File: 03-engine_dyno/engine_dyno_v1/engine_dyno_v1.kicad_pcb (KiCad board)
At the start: 4 copper layers, 92 parts, among them J1 Screw_Terminal_01x02, J2 Screw_Terminal_01x02, J3 Screw_Terminal_01x02, J4 Screw_Terminal_01x05, J5 Screw_Terminal_01x03, J6 Screw_Terminal_01x05, J7 Screw_Terminal_01x03, P1 J1B1211CCD, Q1 PMOS, U1 LMR51430XDDCR, U10 INA827AIDGKR, U11 74LVC1G17, U12 AD630ARZ, U13 ADS1120IPWR, U14 OPA192IDBVR, U15 OPA192IDBVR, U16 74LVC1G17, U2 TVS1800DRV, U3 TPS2115APWR, U4 TPS60403DBVRG4, U5 AD5689RBRUZ, U6 Teensy4.1, U7 INA827AIDGKR, U8 AD630ARZ, U9 ADS1120IPWR

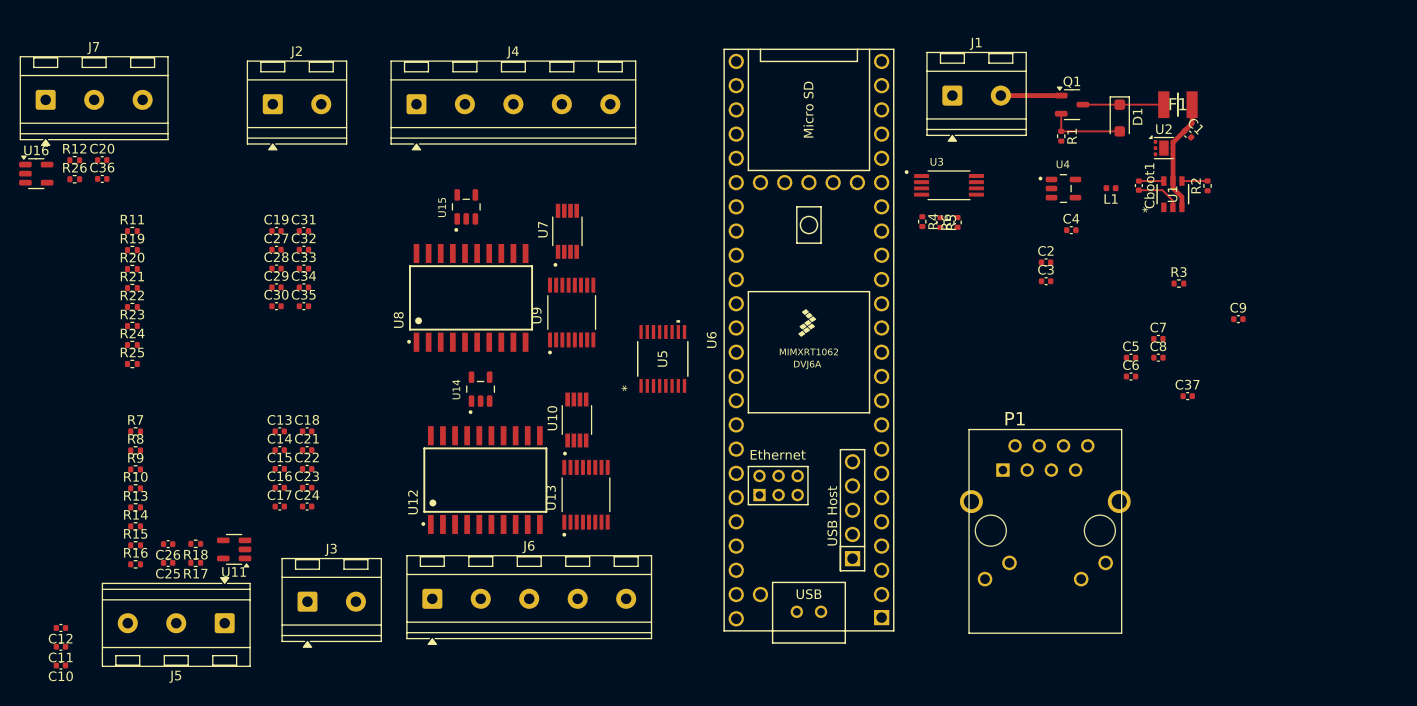
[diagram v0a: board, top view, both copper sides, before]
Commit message: some more changes
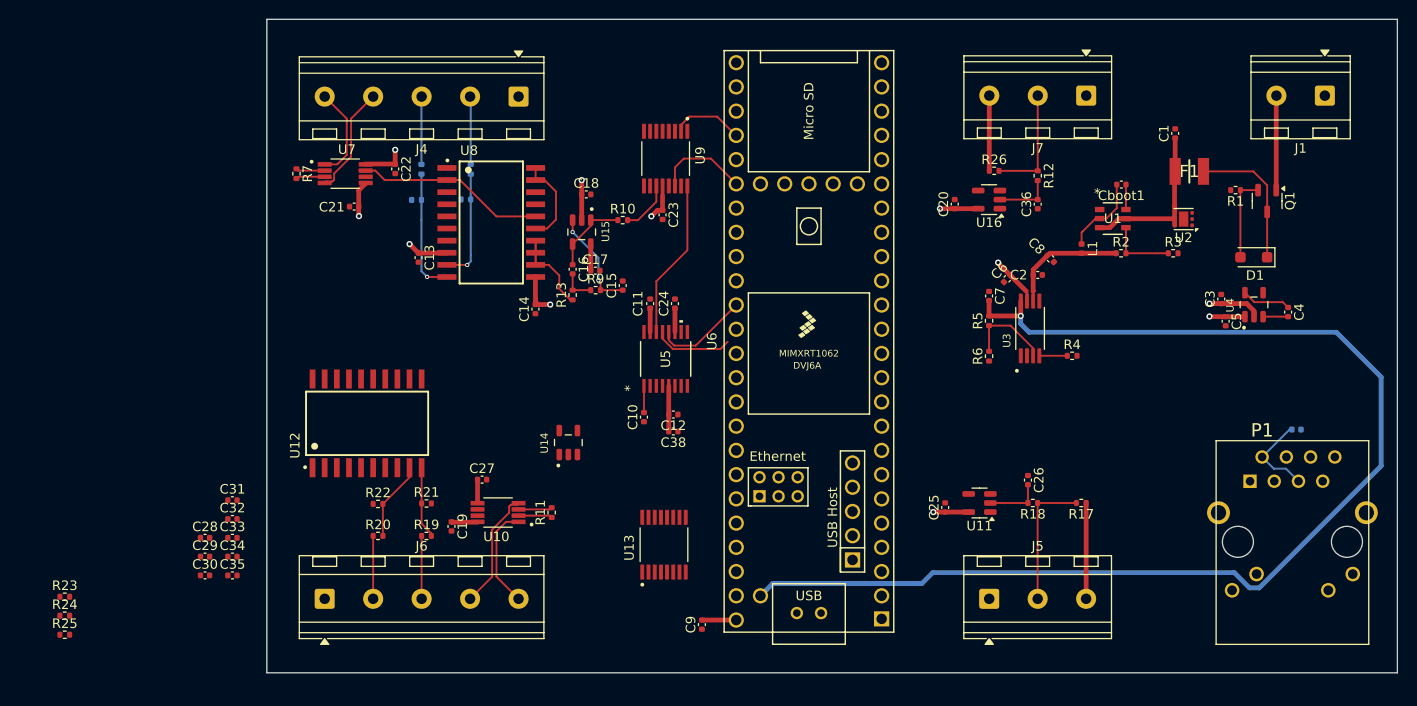
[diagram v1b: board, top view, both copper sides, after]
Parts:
- removed J2, J3: Screw_Terminal_01x02, TerminalBlock_RND:TerminalBlock_RND_205-00232_1x02_P5.08mm_Horizontal
- added C38: 10u, Capacitor_SMD:C_0402_1005Metric, F.Cu at (137.0, 99.0)
- C37, R14, R15, R16, R8: moved to B.Cu
- R11: value 100 -> 390
- R7: value 390 -> 1.5k
- moved J7 109.1 mm to (180.3, 63.8), turned to 180 degrees
- moved R12 101.0 mm to (175.2, 72.2), turned to -90 degrees
- moved U16 99.9 mm to (170.1, 74.7), turned to 180 degrees
- moved C36 98.1 mm to (175.2, 75.2), turned to 90 degrees
- moved R26 96.4 mm to (170.6, 71.7)
- moved R17 93.0 mm to (179.8, 106.5)
- moved C26 90.4 mm to (174.2, 104.1), turned to -90 degrees
- moved C20 89.5 mm to (166.5, 75.2), turned to 90 degrees
- moved R18 87.8 mm to (174.7, 106.5)
- moved C25 81.7 mm to (165.5, 107.0), turned to 90 degrees
- moved J5 80.2 mm to (170.1, 116.5), turned to 0 degrees
- moved U11 78.3 mm to (169.1, 106.5)
- moved C11 71.5 mm to (134.6, 85.6), turned to -90 degrees
- moved C12 68.0 mm to (137.0, 97.2)
- moved C10 66.4 mm to (133.9, 97.5), turned to 90 degrees
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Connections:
- U12 pad 15: /TMNR-5KM/AD630_OUT -> Net-(U12-CH_A-)
- U6 pad 11: unconnected-(U6-9_OUT1C-Pad11) -> /MCU/A16
- U6 pad 12: /MCU/CS_1 -> unconnected-(U6-10_CS_MQSR-Pad12)
- U6 pad 29: /MCU/CS_3 -> unconnected-(U6-37_CS-Pad29)
- U6 pad 31: /MCU/A15 -> unconnected-(U6-39_MISO1_OUT1A-Pad31)
- U6 pad 32: /MCU/A16 -> unconnected-(U6-40_A16-Pad32)
- U6 pad 37: unconnected-(U6-15_A1_RX3_SPDIF_IN-Pad37) -> /MCU/CS_1
- U6 pad 38: /Hall1/HALL -> unconnected-(U6-16_A2_RX4_SCL1-Pad38)
- U6 pad 39: /Hall2/HALL -> unconnected-(U6-17_A3_TX4_SDA1-Pad39)
- U6 pad 4: unconnected-(U6-2_OUT2-Pad4) -> /Hall1/HALL
- U6 pad 44: unconnected-(U6-22_A8_CTX1-Pad44) -> /MCU/A15
- U6 pad 45: unconnected-(U6-23_A9_CRX1_MCLK1-Pad45) -> /MCU/CS_3
- U6 pad 5: unconnected-(U6-3_LRCLK2-Pad5) -> /Hall2/HALL
- U8 pad 15: /Model1605/AD630_OUT -> Net-(U8-CH_A-)
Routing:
- net /MCU/+5V_USB: track 0.00 -> 128.7 mm, vias 0 -> 1
- net +5V: track 0.00 -> 56.1 mm, vias 0 -> 5
- net Net-(U7-VOUT): track 0.00 -> 20.5 mm
- net -5V: track 0.00 -> 18.4 mm, vias 0 -> 4
- net /MCU/MOSI: track 0.00 -> 16.7 mm
- net /Hall2/SIG: track 0.00 -> 14.1 mm
- net Net-(U8-SEL_A): track 0.00 -> 13.1 mm, vias 0 -> 1
- net +3V3: track 0.00 -> 13.0 mm, vias 0 -> 2
- net /TMNR-5KM/SIG+: track 0.00 -> 12.5 mm
- net /power/+5V_BUCK: track 0.00 -> 12.3 mm
- net /Hall1/SIG: track 0.00 -> 11.9 mm
- net Net-(U8-SEL_B): track 0.00 -> 11.8 mm, vias 0 -> 1
- net /Model1605/SIG+: track 0.00 -> 11.5 mm
- net Net-(C15-Pad1): track 0.00 -> 10.9 mm, vias 0 -> 2
- net /TMNR-5KM/SIG-: track 0.00 -> 10.8 mm
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- added copper zone on In2.Cu, net +5V
- added copper zone on In2.Cu, net -5V
- added copper zone on In1.Cu, net GND
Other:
- board outline added: 118.5 x 68.5 mm

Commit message: layout and 3d models
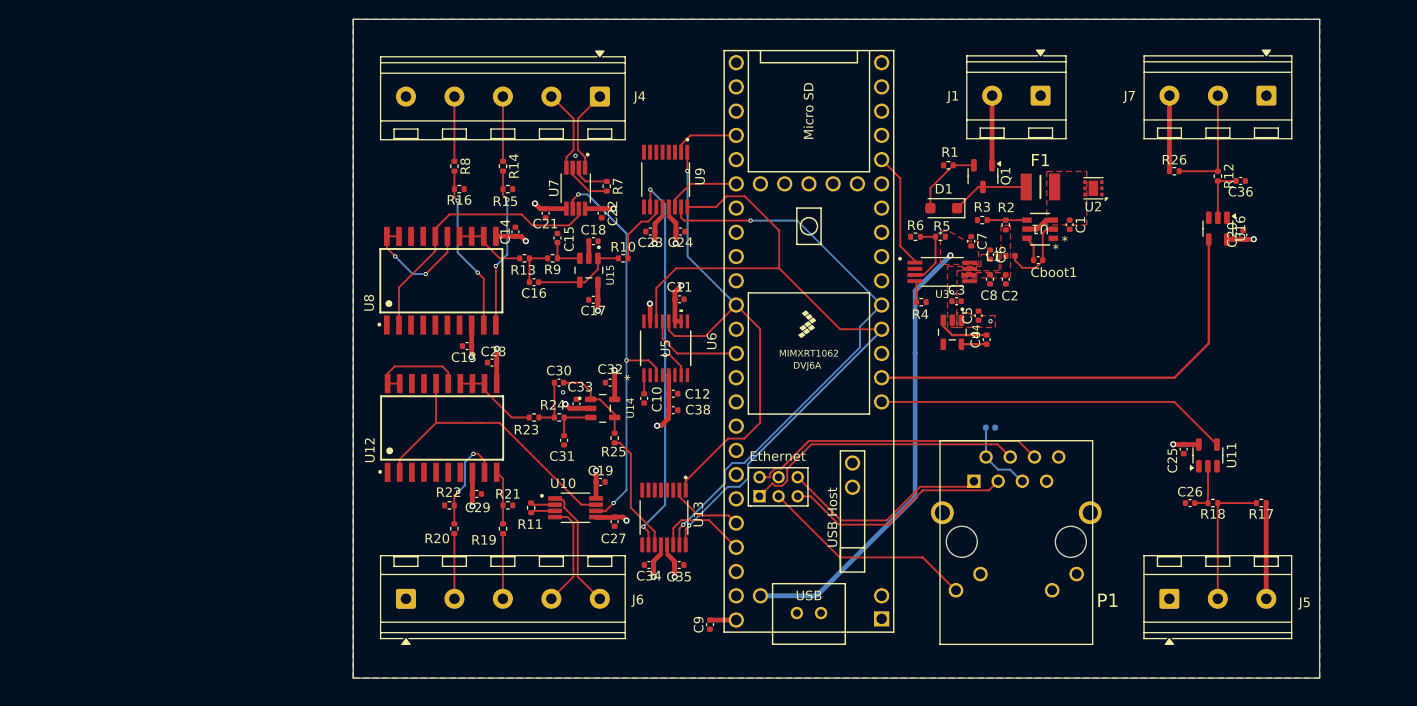
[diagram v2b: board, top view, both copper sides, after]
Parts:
- R14, R15, R16, R8: moved to F.Cu
- moved R25 61.2 mm to (130.9, 99.7), turned to -90 degrees
- moved R24 55.8 mm to (125.0, 97.5)
- moved R23 52.7 mm to (122.4, 97.5)
- moved C35 46.8 mm to (137.6, 113.0)
- moved C34 43.7 mm to (134.4, 113.0), turned to 180 degrees
- moved C30 42.2 mm to (125.0, 93.9), turned to 180 degrees
- moved C32 42.1 mm to (130.4, 93.9), turned to 180 degrees
- moved C33 38.7 mm to (126.8, 96.1), turned to 90 degrees
- moved C31 35.3 mm to (125.6, 99.9), turned to -90 degrees
- moved C28 35.2 mm to (118.0, 91.8)
- moved D1 32.9 mm to (165.3, 75.6)
- moved R7 32.6 mm to (130.0, 73.3)
- moved C37 32.1 mm to (170.2, 98.6)
- moved U4 31.8 mm to (166.2, 88.6), turned to -90 degrees
- moved C4 31.7 mm to (169.8, 89.4), turned to 90 degrees
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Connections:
- net Net-(P1-RD+) renamed /MCU/RD+
- net Net-(P1-RD-) renamed /MCU/RD-
- net Net-(P1-TD+) renamed /MCU/TD+
- net Net-(P1-TD-) renamed /MCU/TD-
- J4 pad 1: /Model1605/CAL -> /Model1605/SIG-
- J4 pad 2: /Model1605/EXC+ -> /Model1605/SIG+
- J4 pad 4: /Model1605/SIG+ -> /Model1605/EXC+
- J4 pad 5: /Model1605/SIG- -> /Model1605/CAL
- U6 pad 10: unconnected-(U6-8_TX2_IN1-Pad10) -> /Hall2/HALL
- U6 pad 11: /MCU/A16 -> /Hall1/HALL
- U6 pad 20: unconnected-(U6-28_RX7-Pad20) -> /MCU/A16
- U6 pad 44: /MCU/A15 -> /MCU/CS_3
- U6 pad 45: /MCU/CS_3 -> /MCU/A15
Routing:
- net /MCU/+5V_USB: track 128.7 -> 47.4 mm
- net /MCU/MOSI: track 16.7 -> 78.0 mm, vias 0 -> 1
- net /MCU/MISO: track 0.00 -> 60.6 mm, vias 0 -> 2
- net /Hall1/HALL: track 0.00 -> 46.7 mm
- net /Model1605/MID_REF: track 0.00 -> 44.0 mm, vias 0 -> 3
- net /Model1605/BIAS_REF: track 0.00 -> 43.8 mm, vias 0 -> 3
- net /MCU/SCK: track 9.93 -> 52.4 mm, vias 0 -> 1
- net /Hall2/HALL: track 0.00 -> 37.0 mm
- net Net-(U10-VOUT): track 0.00 -> 32.2 mm
- net /MCU/RD-: track 0.00 -> 31.3 mm
- net /MCU/RD+: track 0.00 -> 30.1 mm
- net /MCU/TD-: track 0.00 -> 24.9 mm
- net Net-(P1-GRN-): track 0.00 -> 22.7 mm
- net /MCU/TD+: track 0.00 -> 22.1 mm
- net +12V: track 17.5 -> 3.14 mm
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- added copper zone on F.Cu, net +12V
- added copper zone on In2.Cu, net +3V3
- added copper zone on F.Cu, net +5V
- added copper zone on F.Cu, net -5V
- added copper zone on F.Cu, net /MCU/+5V_USB
- added copper zone on F.Cu, net /power/+5V_BUCK
- added copper zone on B.Cu, net GND
- added copper zone on F.Cu, net GND
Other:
- board size 118.5 x 68.5 mm -> 101.3 x 69 mm
